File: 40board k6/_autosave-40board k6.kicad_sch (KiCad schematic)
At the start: 14 parts

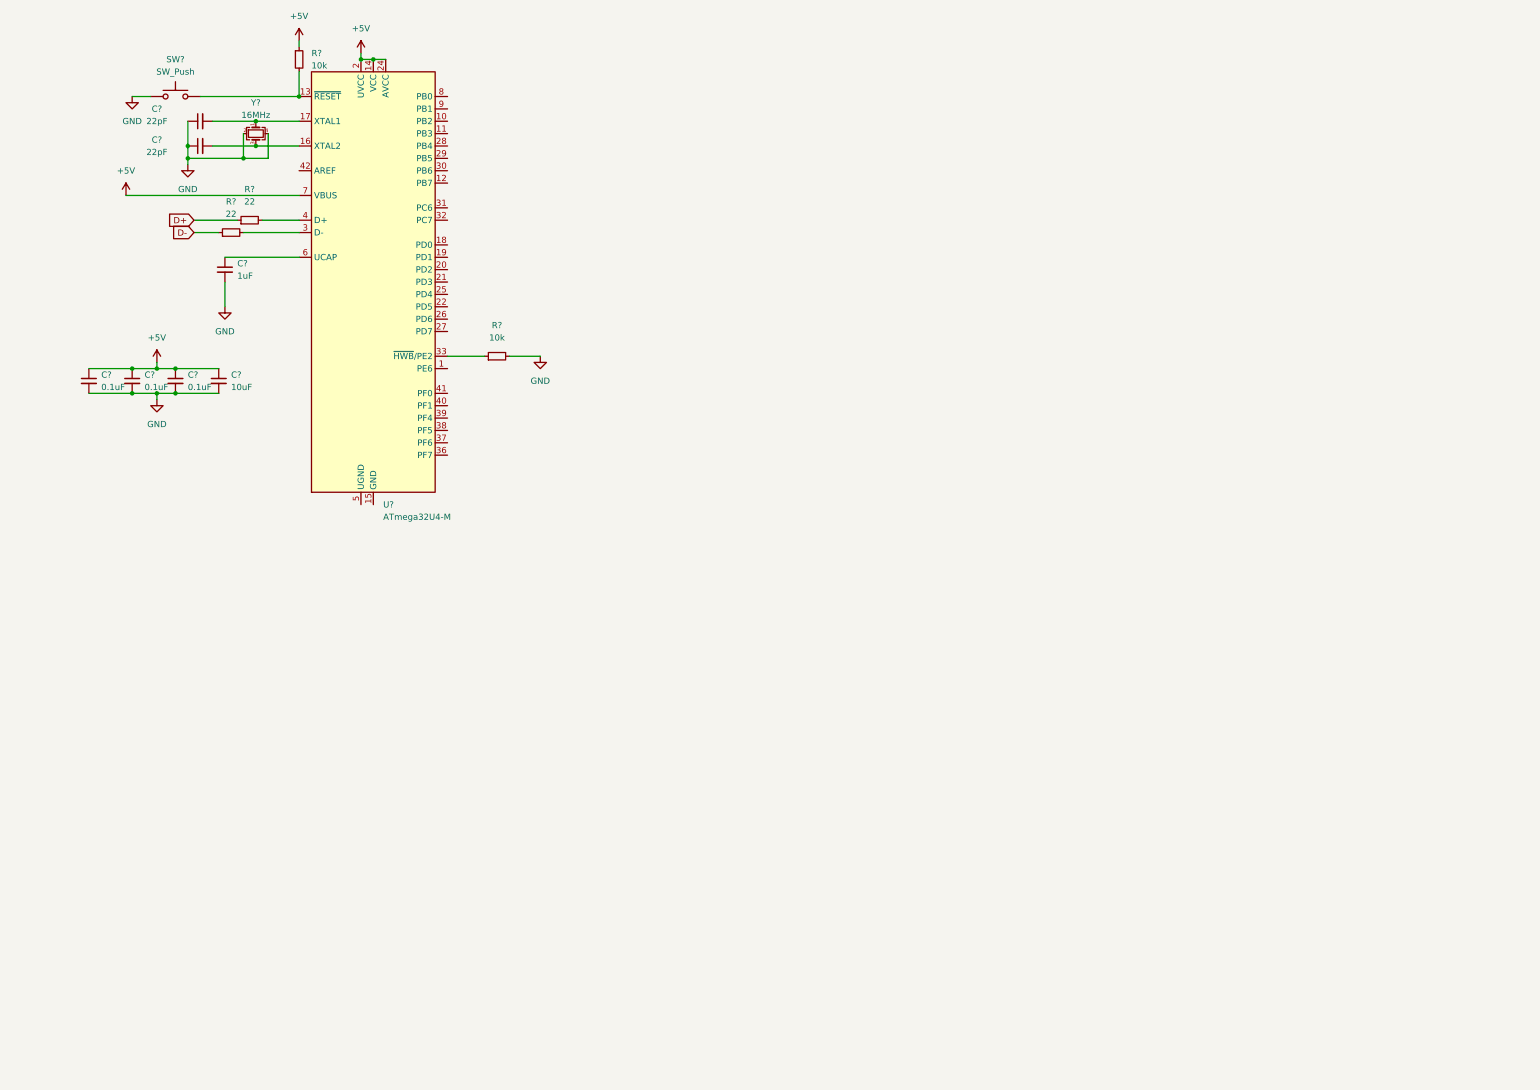
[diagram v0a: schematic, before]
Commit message: Finished Schematic
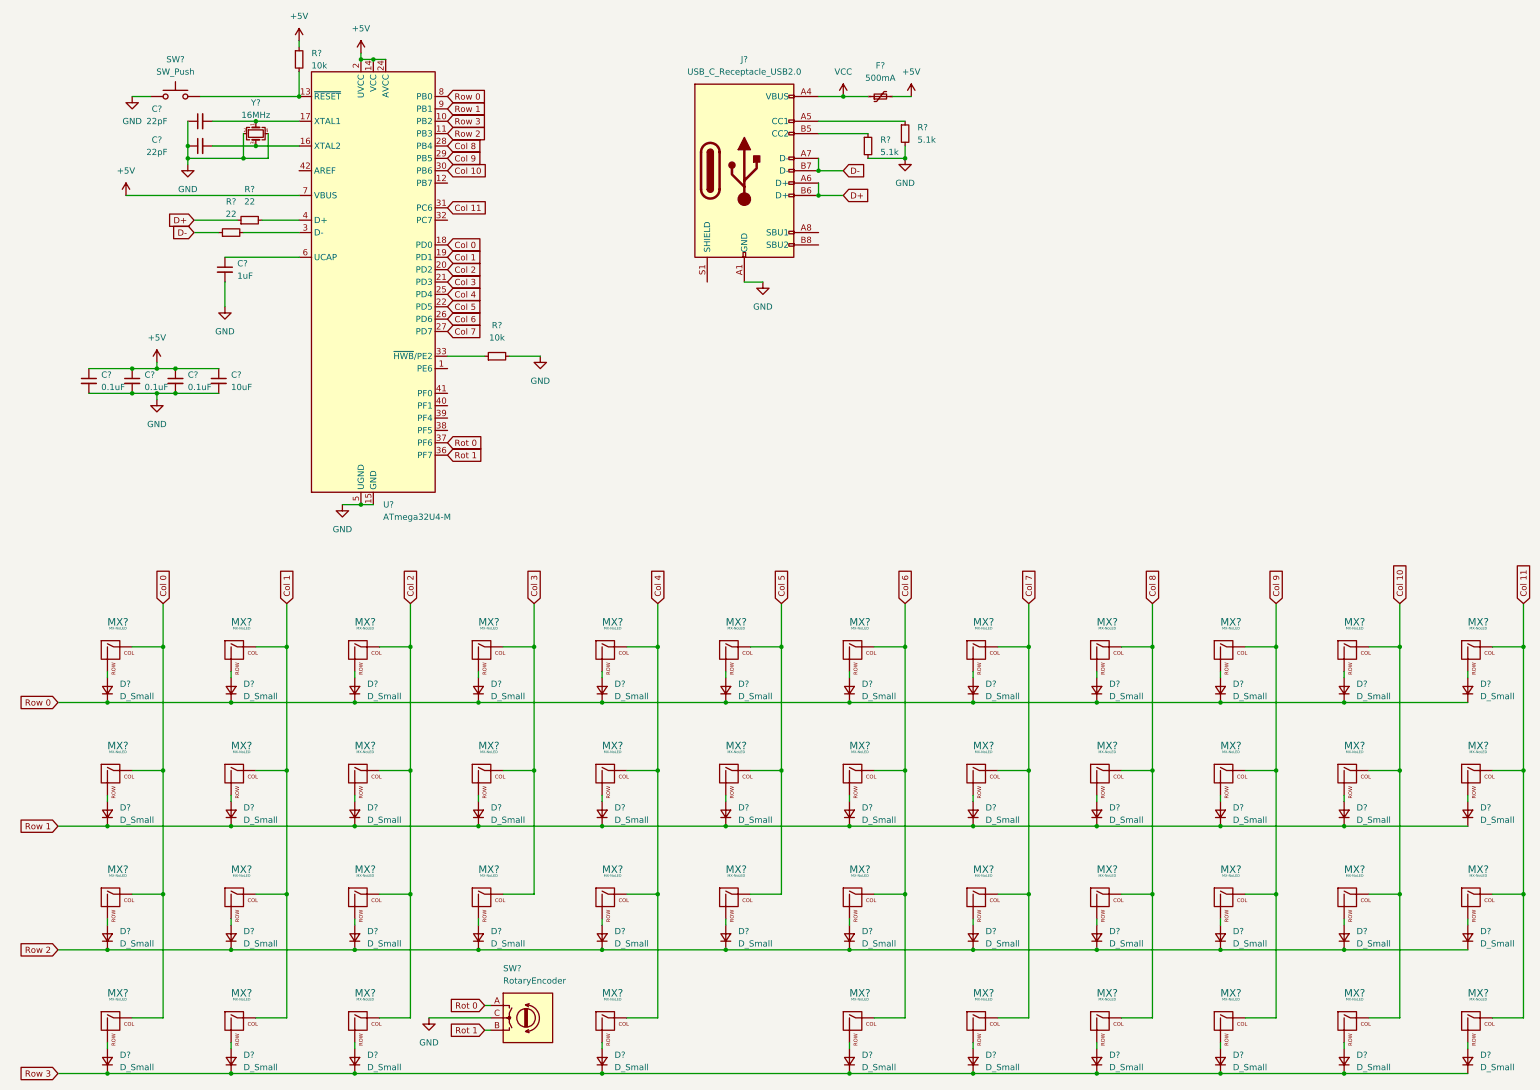
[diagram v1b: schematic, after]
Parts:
- added D? (x46): D_Small, symbol Device:D_Small
- added F?: 500mA, symbol Device:Polyfuse_Small
- added J?: USB_C_Receptacle_USB2.0, symbol Connector:USB_C_Receptacle_USB2.0
- added MX? (x46): MX-NoLED, symbol MX_Alps_Hybrid:MX-NoLED
- added R? (x2): 5.1k, symbol Device:R_Small
- added SW?: RotaryEncoder, symbol Device:RotaryEncoder
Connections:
- net +5V: now also F?.2
- net D+: now also J?.A6 (D+), J?.B6 (D+)
- net D-: now also J?.A7 (D-), J?.B7 (D-)
- net GND: now also U?.15 (GND), U?.23 (GND), U?.35 (GND), U?.43 (GND), U?.45 (GND), U?.5 (UGND), J?.A1 (GND), J?.A12 (GND), J?.B1 (GND), J?.B12 (GND), R?.2, R?.2, SW?.C
- net Row 3: now reaches U?.10 (PB2)
- net Row 3: now also D?.1 (K), D?.1 (K), D?.1 (K), D?.1 (K), D?.1 (K), D?.1 (K), D?.1 (K), D?.1 (K), D?.1 (K), D?.1 (K)
- net Row 2: now reaches U?.11 (PB3)
- net Row 2: now also D?.1 (K), D?.1 (K), D?.1 (K), D?.1 (K), D?.1 (K), D?.1 (K), D?.1 (K), D?.1 (K), D?.1 (K), D?.1 (K), D?.1 (K), D?.1 (K)
- net Col 0: now reaches U?.18 (PD0)
- net Col 0: now also MX?.1 (COL), MX?.1 (COL), MX?.1 (COL), MX?.1 (COL)
- net Col 1: now reaches U?.19 (PD1)
- net Col 1: now also MX?.1 (COL), MX?.1 (COL), MX?.1 (COL), MX?.1 (COL)
- net Col 2: now reaches U?.20 (PD2)
- net Col 2: now also MX?.1 (COL), MX?.1 (COL), MX?.1 (COL), MX?.1 (COL)
- net Col 3: now reaches U?.21 (PD3)
- net Col 3: now also MX?.1 (COL), MX?.1 (COL), MX?.1 (COL)
- net Col 5: now reaches U?.22 (PD5)
- net Col 5: now also MX?.1 (COL), MX?.1 (COL), MX?.1 (COL)
- net Col 4: now reaches U?.25 (PD4)
- net Col 4: now also MX?.1 (COL), MX?.1 (COL), MX?.1 (COL), MX?.1 (COL)
- net Col 6: now reaches U?.26 (PD6)
- net Col 6: now also MX?.1 (COL), MX?.1 (COL), MX?.1 (COL), MX?.1 (COL)
- net Col 7: now reaches U?.27 (PD7)
- net Col 7: now also MX?.1 (COL), MX?.1 (COL), MX?.1 (COL), MX?.1 (COL)
- net Col 8: now reaches U?.28 (PB4)
- net Col 8: now also MX?.1 (COL), MX?.1 (COL), MX?.1 (COL), MX?.1 (COL)
- net Col 9: now reaches U?.29 (PB5)
- net Col 9: now also MX?.1 (COL), MX?.1 (COL), MX?.1 (COL), MX?.1 (COL)
- net Col 10: now reaches U?.30 (PB6)
- net Col 10: now also MX?.1 (COL), MX?.1 (COL), MX?.1 (COL), MX?.1 (COL)
- net Col 11: now reaches U?.31 (PC6)
- net Col 11: now also MX?.1 (COL), MX?.1 (COL), MX?.1 (COL), MX?.1 (COL)
- net Rot 1: now reaches U?.36 (PF7)
- net Rot 1: now also SW?.B
- net Rot 0: now reaches U?.37 (PF6)
- net Rot 0: now also SW?.A
- net Row 0: now reaches U?.8 (PB0)
- net Row 0: now also D?.1 (K), D?.1 (K), D?.1 (K), D?.1 (K), D?.1 (K), D?.1 (K), D?.1 (K), D?.1 (K), D?.1 (K), D?.1 (K), D?.1 (K), D?.1 (K)
- net Row 1: now reaches U?.9 (PB1)
- net Row 1: now also D?.1 (K), D?.1 (K), D?.1 (K), D?.1 (K), D?.1 (K), D?.1 (K), D?.1 (K), D?.1 (K), D?.1 (K), D?.1 (K), D?.1 (K), D?.1 (K)
- new net: D?.2 (A), MX?.2 (ROW) (x46)
- new net: J?.A5 (CC1), R?.1
- new net: J?.B5 (CC2), R?.1
- new net VCC: F?.1, J?.A4 (VBUS), J?.A9 (VBUS), J?.B4 (VBUS), J?.B9 (VBUS)
